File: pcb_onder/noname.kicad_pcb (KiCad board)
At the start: 2 copper layers, 18 parts

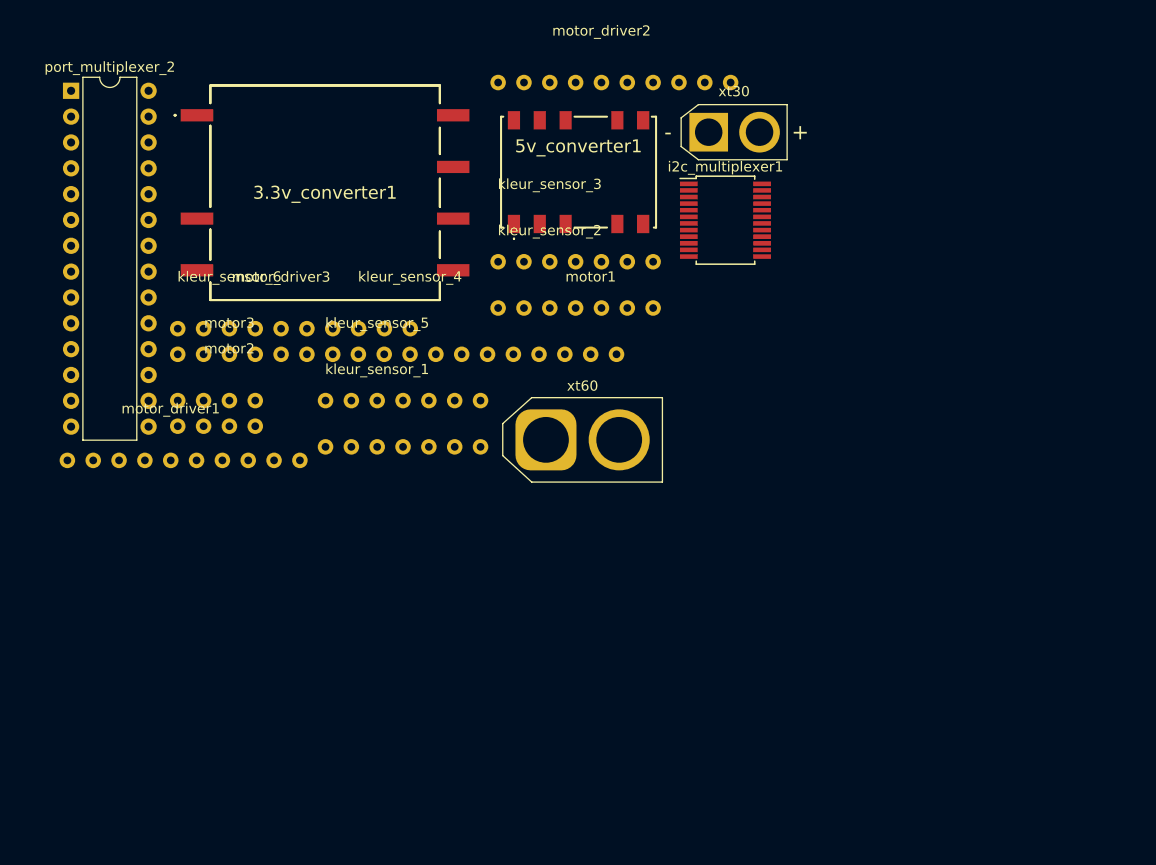
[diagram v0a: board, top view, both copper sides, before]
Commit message: pcb onder gemaakt
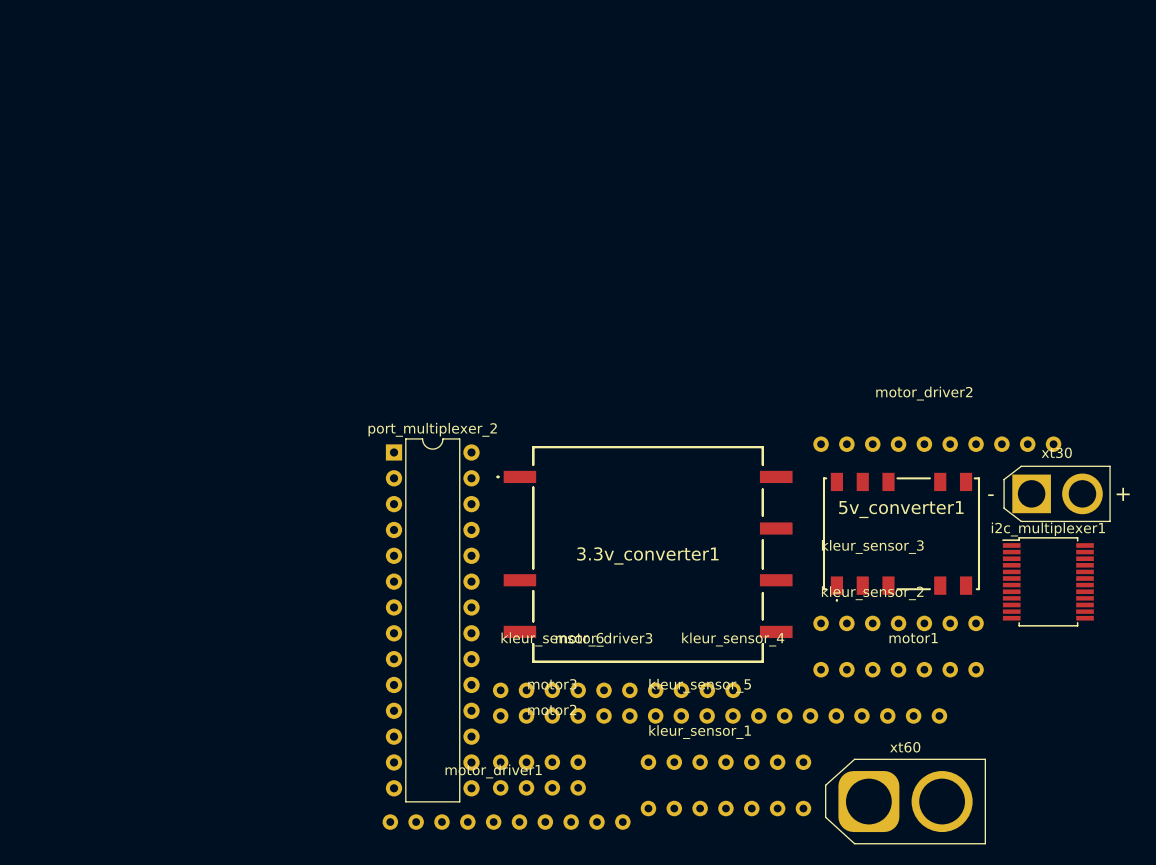
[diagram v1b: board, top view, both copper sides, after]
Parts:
- moved motor_driver1 47.7 mm to (150.6, 158.6)
- moved kleur_sensor_2 47.7 mm to (187.9, 146.1)
- moved xt60 47.7 mm to (187.5, 156.5)
- moved 3.3v_converter1 47.7 mm to (165.8, 132.3)
- moved 5v_converter1 47.7 mm to (190.7, 130.2)
- moved kleur_sensor_3 47.7 mm to (187.9, 141.6)
- moved kleur_sensor_4 47.7 mm to (174.2, 150.7)
- moved kleur_sensor_5 47.7 mm to (170.9, 155.2)
- moved kleur_sensor_6 47.7 mm to (156.4, 150.7)
- moved motor1 47.7 mm to (191.9, 148.1)
- moved motor2 47.7 mm to (156.4, 155.2)
- moved motor_driver2 47.7 mm to (193.0, 121.4)
- moved xt30 47.7 mm to (203.5, 126.3)
- moved i2c_multiplexer1 47.7 mm to (205.2, 134.9)
- moved kleur_sensor_1 47.7 mm to (170.9, 159.8)
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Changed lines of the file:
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@@
       (creategerberjobfile true)
       (excludeedgelayer true)
-      (linewidth 0.100000)
+      (linewidth 0.150000)
       (plotframeref false)
       (viasonmask false)
@@
   )
   (module Connector_AMASS:AMASS_XT60-F_1x02_P7.20mm_Vertical (layer F.Cu)
-    (at 155.765001 120.985001)
+    (at 187.515001 156.545001)
     (descr "AMASS female XT60, through hole, vertical, https://www.tme.eu/Document/2d152ced3b7a446066e6c419d84bb460/XT60%20SPEC.pdf")
     (tags "XT60 female vertical")
@@
   )
   (module Connector_AMASS:AMASS_XT30U-F_1x02_P5.0mm_Vertical (layer F.Cu)
-    (at 171.765001 90.735001)
+    (at 203.515001 126.295001)
     (descr "Connector XT30 Vertical Cable Female, https://www.tme.eu/en/Document/3cbfa5cfa544d79584972dd5234a409e/XT30U%20SPEC.pdf")
     (tags "RC Connector XT30")
@@
   )
   (module Package_DIP:DIP-28_W7.62mm (layer F.Cu)
-    (at 109.075001 86.665001)
+    (at 140.825001 122.225001)
     (descr "28-lead though-hole mounted DIP package, row spacing 7.62 mm (300 mils)")
     (tags "THT DIP DIL PDIP 2.54mm 7.62mm 300mil")
@@
   )
   (module custom:TB9051FTG (layer F.Cu)
-    (at 129.722 110.052)
+    (at 161.472 145.612)
     (fp_text reference motor_driver3 (at 0 -5.08) (layer F.SilkS)
       (effects (font (size 1 1) (thickness 0.15)))
@@
   )
   (module custom:TB9051FTG (layer F.Cu)
-    (at 161.222 85.852)
+    (at 192.972 121.412)
     (fp_text reference motor_driver2 (at 0 -5.08) (layer F.SilkS)
       (effects (font (size 1 1) (thickness 0.15)))
@@
   )
   (module custom:TB9051FTG (layer F.Cu)
-    (at 118.872 123.002)
+    (at 150.622 158.562)
     (fp_text reference motor_driver1 (at 0 -5.08) (layer F.SilkS)
       (effects (font (size 1 1) (thickness 0.15)))
@@
   )
   (module custom:pololu_motor (layer F.Cu)
-    (at 124.642 117.122)
+    (at 156.392 152.682)
     (fp_text reference motor3 (at 0 -7.62) (layer F.SilkS)
       (effects (font (size 1 1) (thickness 0.15)))
@@
   )
   (module custom:pololu_motor (layer F.Cu)
-    (at 124.642 119.642)
+    (at 156.392 155.202)
     (fp_text reference motor2 (at 0 -7.62) (layer F.SilkS)
       (effects (font (size 1 1) (thickness 0.15)))
@@
   )
   (module custom:pololu_motor (layer F.Cu)
-    (at 160.162 112.572)
+    (at 191.912 148.132)
     (fp_text reference motor1 (at 0 -7.62) (layer F.SilkS)
       (effects (font (size 1 1) (thickness 0.15)))
@@
   )
   (module custom:tcs3472 (layer F.Cu)
-    (at 124.642 115.112)
+    (at 156.392 150.672)
     (fp_text reference kleur_sensor_6 (at 0 -10.16) (layer F.SilkS)
       (effects (font (size 1 1) (thickness 0.15)))
@@
   )
   (module custom:tcs3472 (layer F.Cu)
-    (at 139.172 119.662)
+    (at 170.922 155.222)
     (fp_text reference kleur_sensor_5 (at 0 -10.16) (layer F.SilkS)
       (effects (font (size 1 1) (thickness 0.15)))
@@
   )
   (module custom:tcs3472 (layer F.Cu)
-    (at 142.402 115.112)
+    (at 174.152 150.672)
     (fp_text reference kleur_sensor_4 (at 0 -10.16) (layer F.SilkS)
       (effects (font (size 1 1) (thickness 0.15)))
@@
   )
   (module custom:tcs3472 (layer F.Cu)
-    (at 156.142 106.012)
+    (at 187.892 141.572)
     (fp_text reference kleur_sensor_3 (at 0 -10.16) (layer F.SilkS)
       (effects (font (size 1 1) (thickness 0.15)))
@@
   )
   (module custom:tcs3472 (layer F.Cu)
-    (at 156.142 110.562)
+    (at 187.892 146.122)
     (fp_text reference kleur_sensor_2 (at 0 -10.16) (layer F.SilkS)
       (effects (font (size 1 1) (thickness 0.15)))
@@
   )
   (module custom:tcs3472 (layer F.Cu)
-    (at 139.172 124.212)
+    (at 170.922 159.772)
     (fp_text reference kleur_sensor_1 (at 0 -10.16) (layer F.SilkS)
       (effects (font (size 1 1) (thickness 0.15)))
@@
   )
   (module Package_SO:SSOP-24_5.3x8.2mm_P0.65mm (layer F.Cu)
-    (at 173.415001 99.385001)
+    (at 205.165001 134.945001)
     (descr "24-Lead Plastic Shrink Small Outline (SS)-5.30 mm Body [SSOP] (see Microchip Packaging Specification 00000049BS.pdf)")
     (tags "SSOP 0.65")
@@
   )
   (module custom:SFTN01M05N (layer F.Cu)
-    (at 158.970001 94.660001)
+    (at 190.720001 130.220001)
     (descr SFTN01M-05N-2)
     (tags "Power Supply")
@@
   )
   (module custom:CC60512SRE (layer F.Cu)
-    (at 134.050001 96.690001)
+    (at 165.800001 132.250001)
     (descr CC6-0512SR-E-4)
     (tags "Power Supply")
